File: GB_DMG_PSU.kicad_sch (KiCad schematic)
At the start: 33 parts, among them J1 Conn_01x02, J2 Conn_01x04, J3 Conn_01x02, Q1 BSS84, U1 R1283K001C-TR, U4 MCP73831

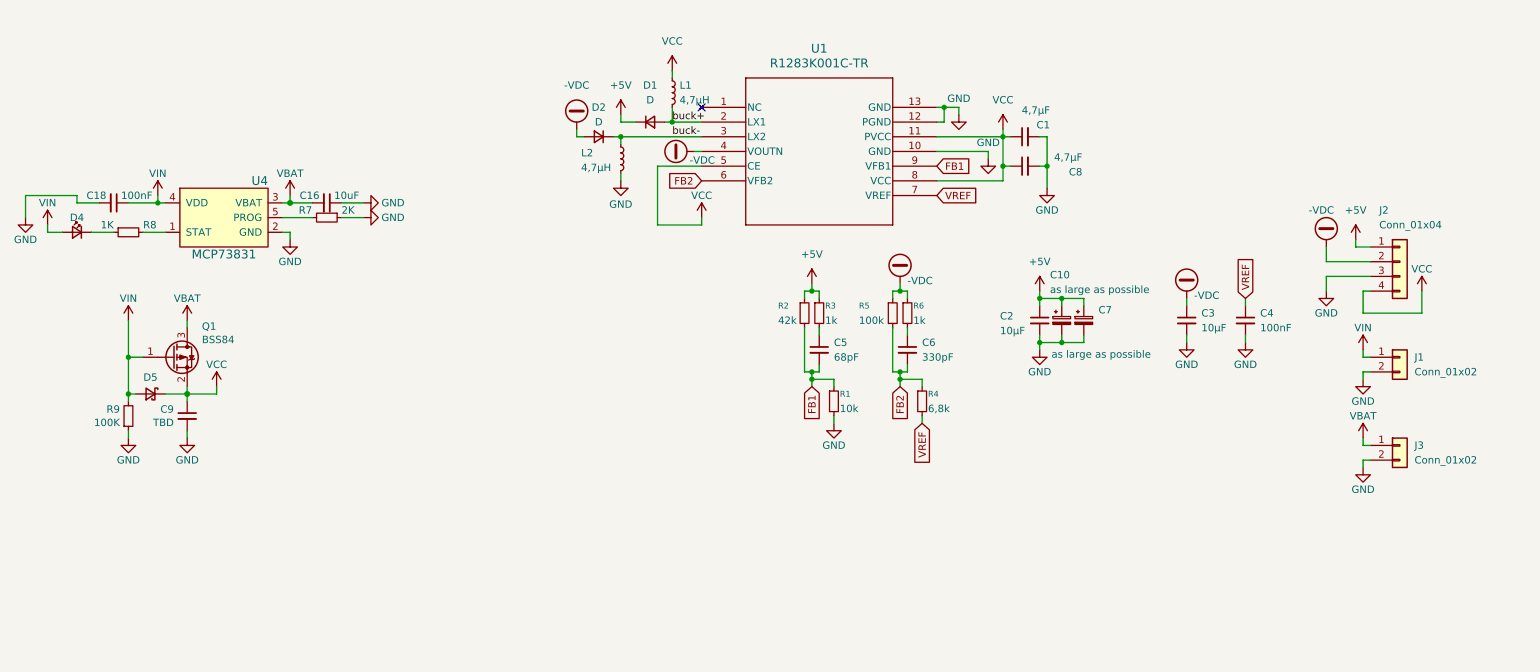
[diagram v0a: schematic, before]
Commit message: V2
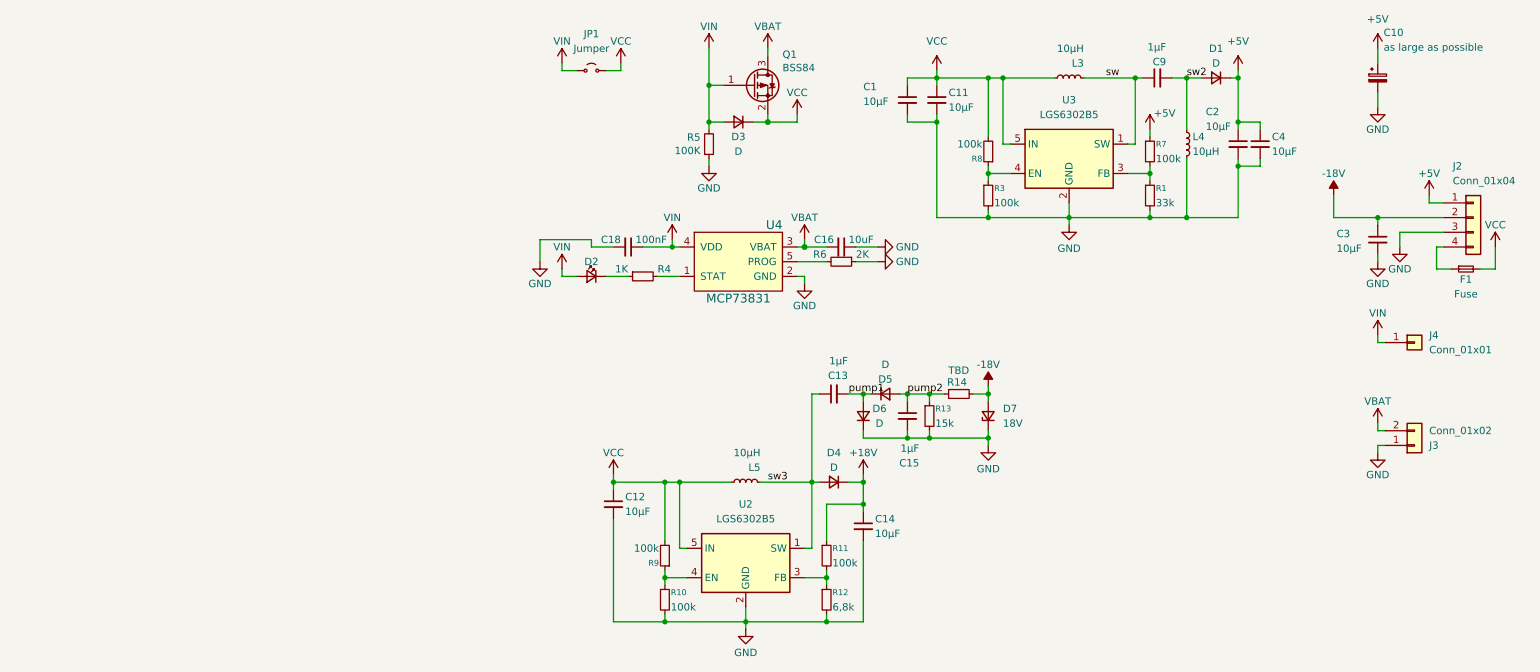
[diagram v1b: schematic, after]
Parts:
- removed C5: 68pF, Capacitor_SMD:C_0603_1608Metric, symbol Device:C_Small
- removed C6: 330pF, Capacitor_SMD:C_0603_1608Metric, symbol Device:C_Small
- removed C7: as large as possible, Capacitor_Tantalum_SMD:CP_EIA-3528-12_Kemet-T, symbol Device:C_Polarized_Small
- removed C8: 4,7µF, Capacitor_SMD:C_0603_1608Metric, symbol Device:C_Small
- removed D2: D, Diode_SMD:D_SOD-323, symbol Device:D_Small
- removed D4: LED_CHR, LED_SMD:LED_0402_1005Metric, symbol Device:LED_Small
- removed D5: D_Schottky_Small, Diode_SMD:D_SOD-323, symbol Device:D_Schottky_Small
- removed J1: Conn_01x02, symbol Connector_Generic:Conn_01x02
- removed L1, L2: 4,7µH, Inductor_SMD:L_0805_2012Metric, symbol Device:L_Small
- removed R2: 42k, Resistor_SMD:R_0603_1608Metric, symbol Device:R_Small
- removed U1: R1283K001C-TR, footprints:PE-DFNPL2730-12-180404_NMD, symbol 2025-10-09_16-12-42:R1283K001C-TR
- added C11, C12, C14: 10µF, Capacitor_SMD:C_0603_1608Metric, symbol Device:C_Small
- added C13, C15: 1µF, Capacitor_SMD:C_0603_1608Metric, symbol Device:C_Small
- added D2: LED_CHR, LED_THT:LED_D3.0mm, symbol Device:LED_Small
- added D3, D4, D5, D6: D, Diode_SMD:D_SOD-323, symbol Device:D_Small
- added D7: 18V, Diode_SMD:D_SOD-323, symbol Device:D_Zener_Small
- added F1: Fuse, Fuse:Fuse_1206_3216Metric, symbol Device:Fuse_Small
- added J4: Conn_01x01, Connector_PinHeader_2.54mm:PinHeader_1x01_P2.54mm_Vertical, symbol Connector_Generic:Conn_01x01
- added JP1: Jumper, Jumper:SolderJumper-2_P1.3mm_Open_RoundedPad1.0x1.5mm, symbol Jumper:Jumper_2_Small_Open
- added L3, L4, L5: 10µH, Inductor_SMD:L_APV_ANR5040, symbol Device:L_Small
- added R10, R11: 100k, Resistor_SMD:R_0603_1608Metric, symbol Device:R_Small
- added R12: 6,8k, Resistor_SMD:R_0603_1608Metric, symbol Device:R_Small
- added R13: 15k, Resistor_SMD:R_0603_1608Metric, symbol Device:R_Small
- added R14: TBD, Resistor_SMD:R_0603_1608Metric, symbol Device:R_Small
- added U2, U3: LGS6302B5, Package_TO_SOT_SMD:SOT-23-5, symbol Regulator_Switching:LGS6302B5
- C1: value 4,7µF -> 10µF
- C18: footprint Capacitor_SMD:C_0402_1005Metric -> Capacitor_SMD:C_0603_1608Metric
- C3: footprint Capacitor_SMD:C_0603_1608Metric -> Capacitor_SMD:C_1206_3216Metric
- C4: value 100nF -> 10µF
- C9: value TBD -> 1µF; footprint Capacitor_SMD:C_0402_1005Metric -> Capacitor_SMD:C_0603_1608Metric
- J3: footprint (none) -> Connector_JST:JST_PH_S2B-PH-K_1x02_P2.00mm_Horizontal
- R1: value 10k -> 33k
- R3: value 1k -> 100k
- R4: value 6,8k -> 1K
- R5: value 100k -> 100K
- R6: value 1k -> 2K
- R7: value 2K -> 100k; footprint Resistor_SMD:R_0402_1005Metric -> Resistor_SMD:R_0603_1608Metric
- R8: value 1K -> 100k; footprint Resistor_SMD:R_0402_1005Metric -> Resistor_SMD:R_0603_1608Metric
- R9: value 100K -> 100k; footprint Resistor_SMD:R_0402_1005Metric -> Resistor_SMD:R_0603_1608Metric
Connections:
- net +5V: now also C4.1, R7.1; no longer R3.1
- net GND: now also J3.1 (Pin_1), R3.2, R5.1, R6.1, C11.2, C12.2, C14.2, C15.2, D6.1 (K), D7.1 (K), L4.2, R10.2, R12.2, R13.2, U2.2 (GND), U3.2 (GND); no longer C9.2, J3.2 (Pin_2), R7.1, R9.1
- net VBAT: now also J3.2 (Pin_2); no longer J3.1 (Pin_1)
- net VCC: now also R8.2, R9.2, C11.1, C12.1, D3.1 (K), F1.2, JP1.2 (B), L3.1, L5.1, U2.5 (IN), U3.5 (IN); no longer C9.1, J2.4 (Pin_4)
- net VIN: now also R5.2, D2.2 (A), D3.2 (A), J4.1 (Pin_1), JP1.1 (A); no longer R9.2
- net at R8.1: now also R3.1, U3.4 (EN)
- net at U4.1 (STAT): now also R4.2; no longer R8.2
- net at U4.5 (PROG): now also R6.2; no longer R7.2
- net -VDC renamed -18V
- net -18V: now also D7.2 (A), R14.2; no longer R5.1, R6.1
- net FB1: no longer names the net of R1.1
- net FB1: now also R7.2, U3.3 (FB)
- net FB2: no longer names the net of R4.1
- net FB2: now also D2.1 (K); no longer R5.2
- removed net VREF: C4.1, R4.2
- net buck+ renamed sw2
- net sw2: now also C9.2, L4.1
- new net: F1.1, J2.4 (Pin_4)
- new net: R11.2, R12.1, U2.3 (FB)
- new net: R10.1, R9.1, U2.4 (EN)
- new net +18V: C14.1, D4.1 (K), R11.1
- new net pump1: C13.2, D5.1 (K), D6.2 (A)
- new net pump2: C15.1, D5.2 (A), R13.1, R14.1
- new net sw: C9.1, L3.2, U3.1 (SW)
- new net sw3: C13.1, D4.2 (A), L5.2, U2.1 (SW)
- no-connect marks 1 -> 0
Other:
- moved on the sheet: C10, C16, C18, C2, C3, D1, J2, J3, Q1, R1, R3, U4
